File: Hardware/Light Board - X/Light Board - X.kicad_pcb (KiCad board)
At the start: 2 copper layers, 51.7 x 38.4 mm, 12 parts, among them J1 V+, J2 V-

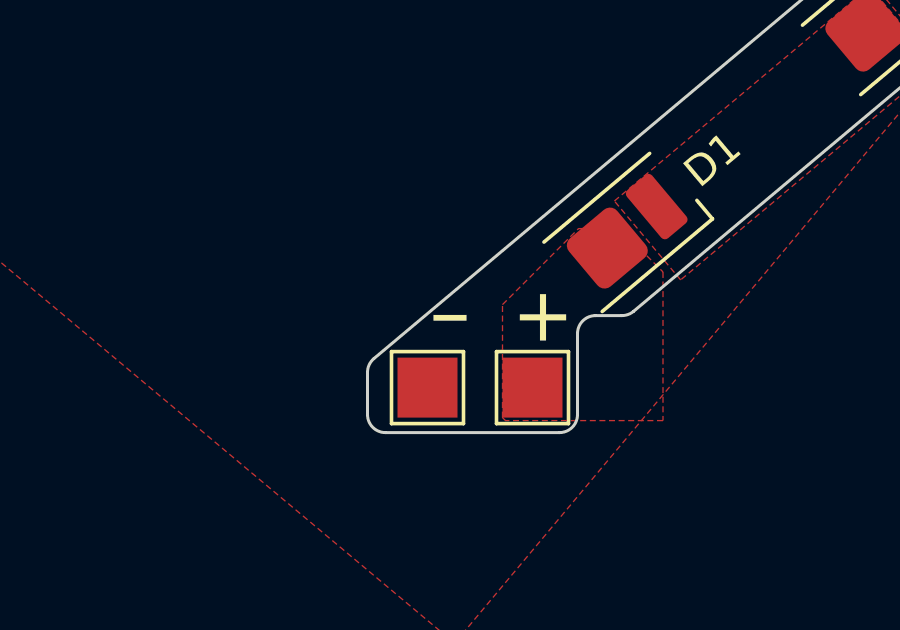
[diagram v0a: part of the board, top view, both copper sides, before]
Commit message: Finished all light boards
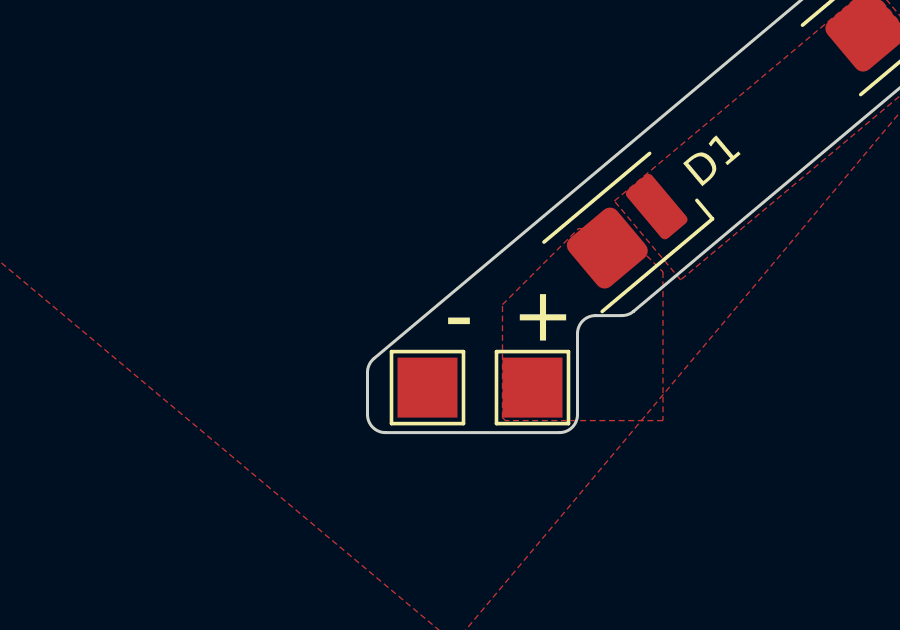
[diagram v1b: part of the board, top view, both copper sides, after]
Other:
- board text added: "-"
- board text removed: "–"
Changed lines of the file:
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@@
 		)
 	)
-	(gr_text "–"
-		(at 125.3 123.8 0)
+	(gr_text "-"
+		(at 125.6 123.9 0)
 		(layer "F.SilkS")
 		(effects
